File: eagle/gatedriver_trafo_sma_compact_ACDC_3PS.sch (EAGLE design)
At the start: 34 parts, among them K1 G5V-2, X4 BU-SMA-V

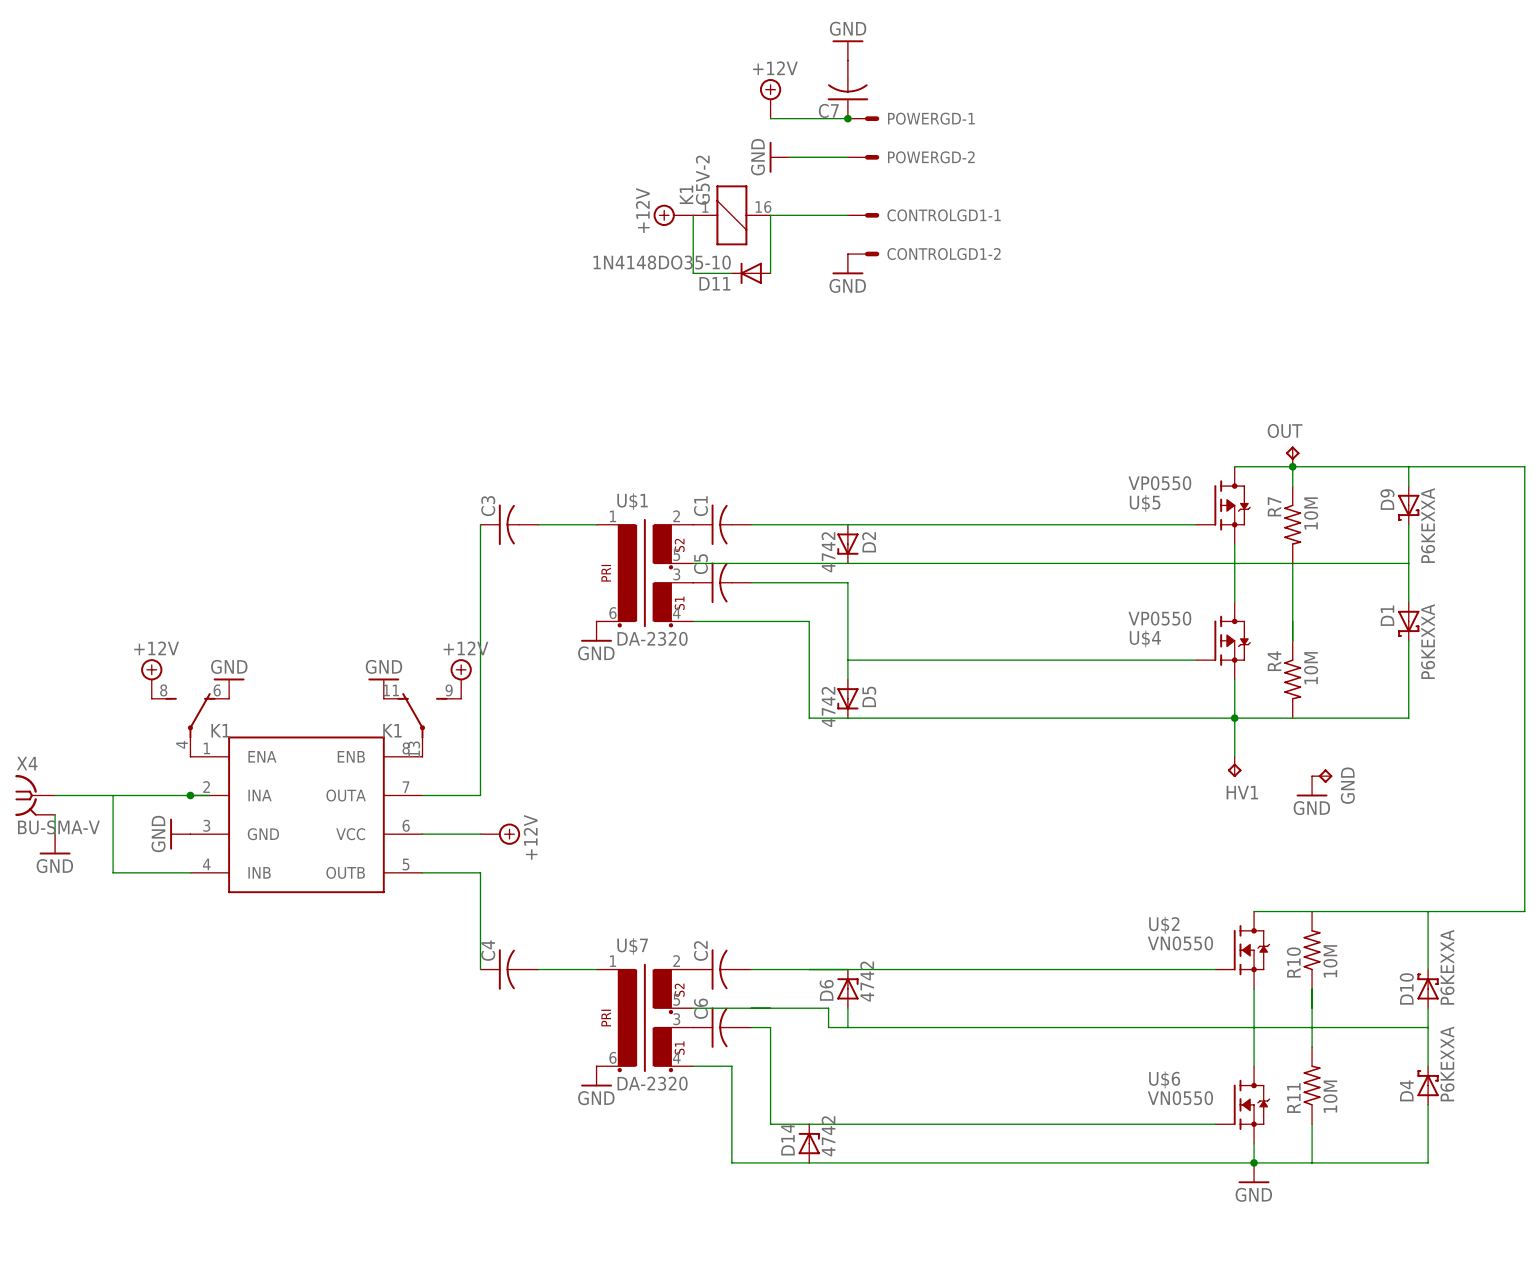
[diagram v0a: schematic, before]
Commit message: IXYS board solution, gatedriver components
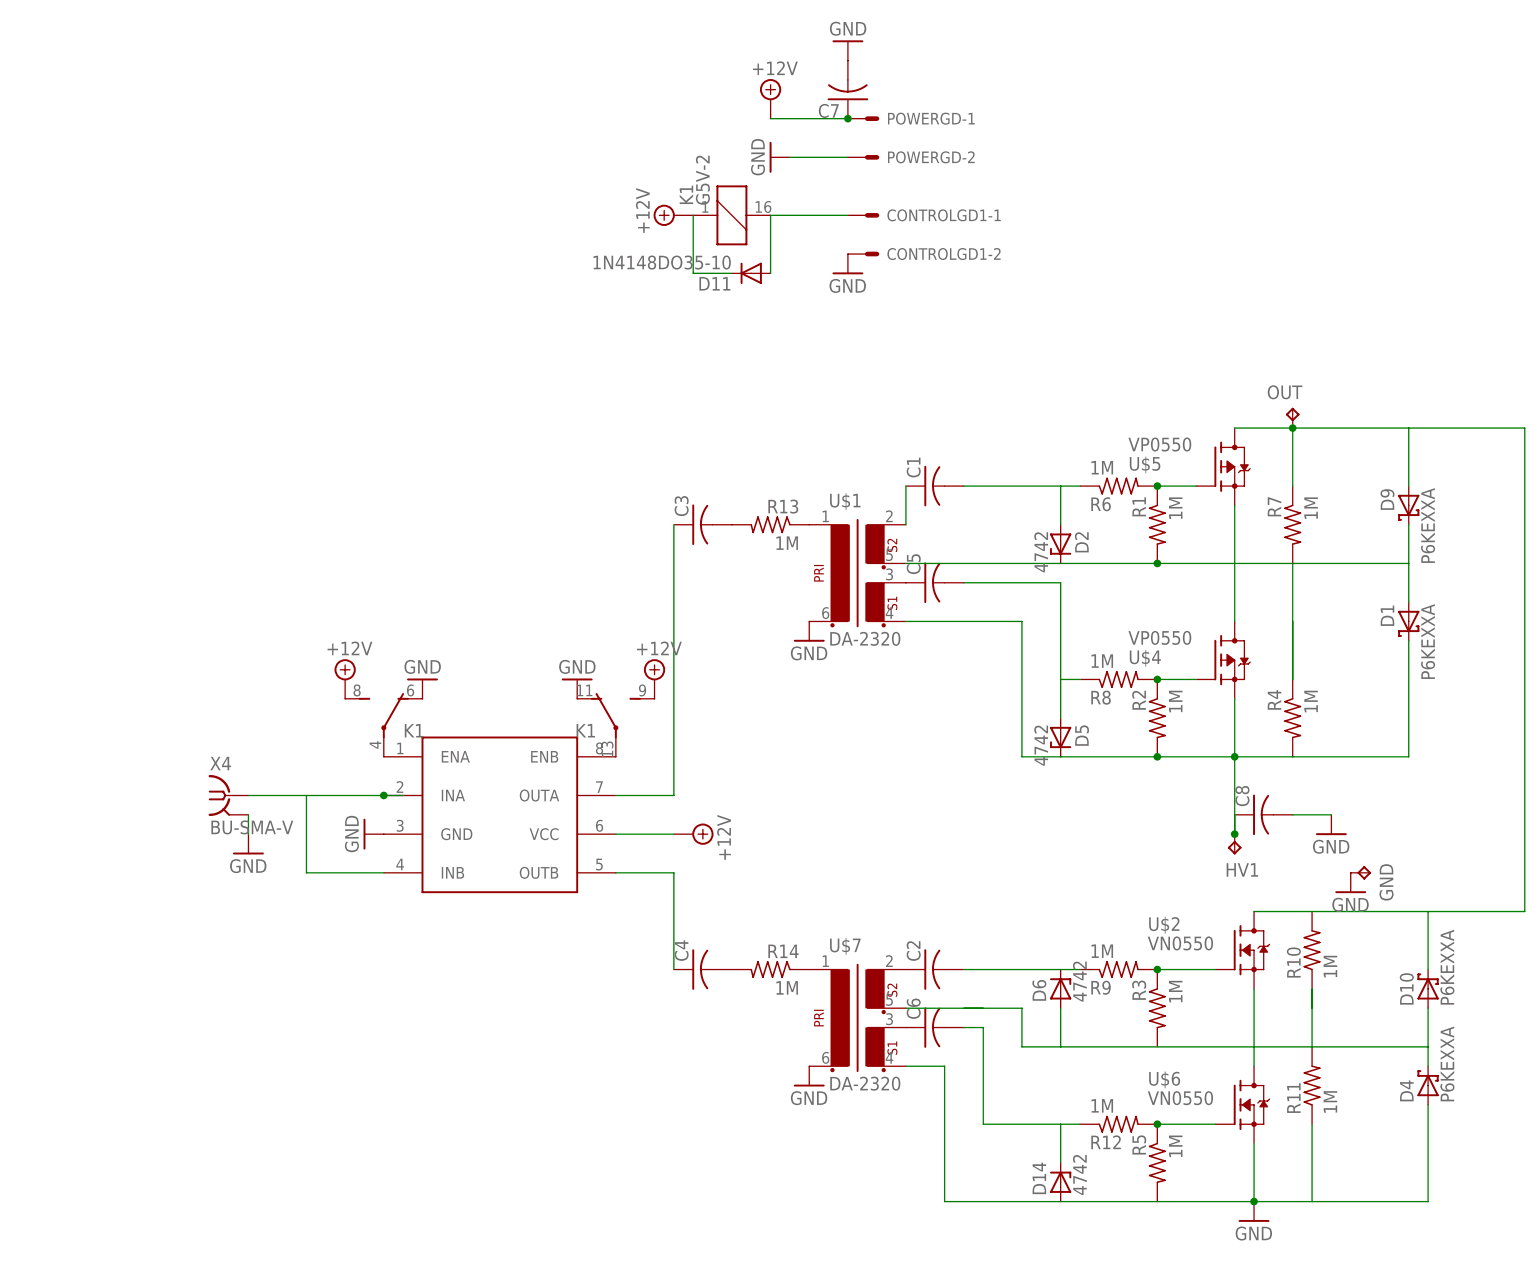
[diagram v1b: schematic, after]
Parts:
- added C8: (no value), resistor:C-US102-064X133
- added R1, R12, R2, R3, R5, R6, R8, R9: 1M, rcl:R-US_0207/10
- added R13, R14: 1M, rcl:R-US_0207/12
- R10, R11, R4, R7: value 10M -> 1M; device rcl:R-US_0207/12 -> rcl:R-US_0207/10
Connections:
- new net N$10: C1.2, D2.A, R6.1
- new net N$12: R2.1, R8.2, U$4.G
- new net N$19: C3.2, R13.2
- new net N$20: C4.2, R14.2
- new net N$8: R1.1, R6.2, U$5.G
- net GND: now also C8.2
- net N$11: now also R12.2, R5.1, U$6.G; no longer C1.2, D2.A, U$5.G
- net N$16: now also R8.1; no longer U$4.G
- net N$17: now also C8.1, R2.2
- net N$18: now also R1.2
- net N$25: now also R3.1, R9.1, R9.2
- net N$27: now also R12.1; no longer U$6.G
- net N$3: now also R13.1; no longer C3.2
- net N$6: now also R14.1; no longer C4.2
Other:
- moved on the sheet: C1, C2, C3, C4, C5, C6, D14, D2, D5, D6, GND, HV1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
